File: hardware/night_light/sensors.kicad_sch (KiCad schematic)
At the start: 6 parts, among them J1 RDB223

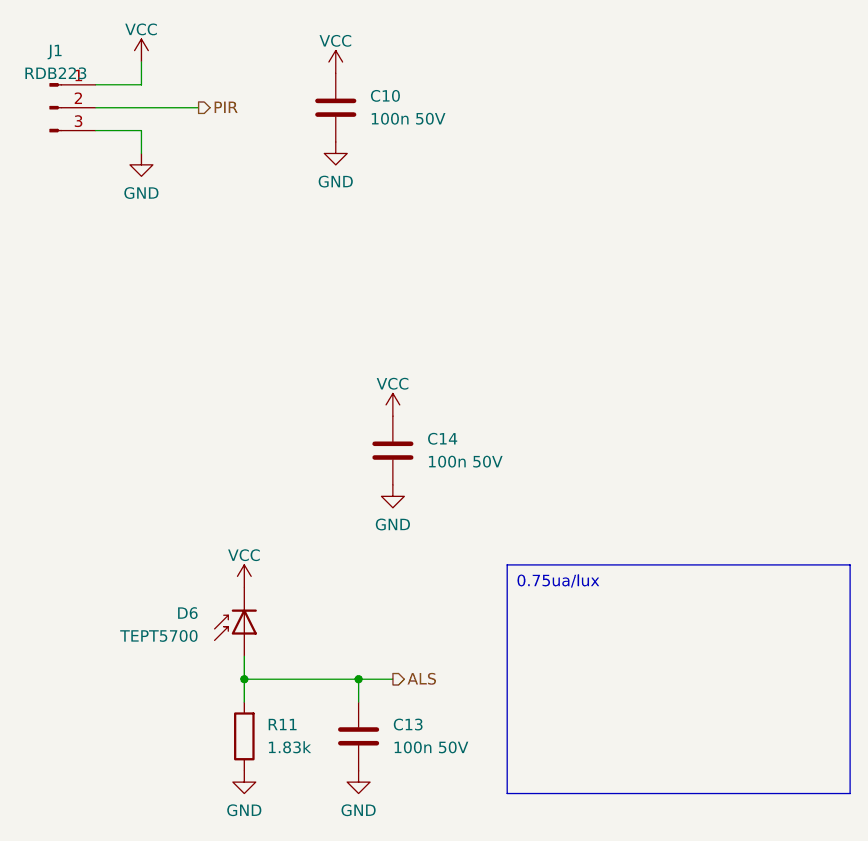
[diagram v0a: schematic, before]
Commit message: Night Light firmware
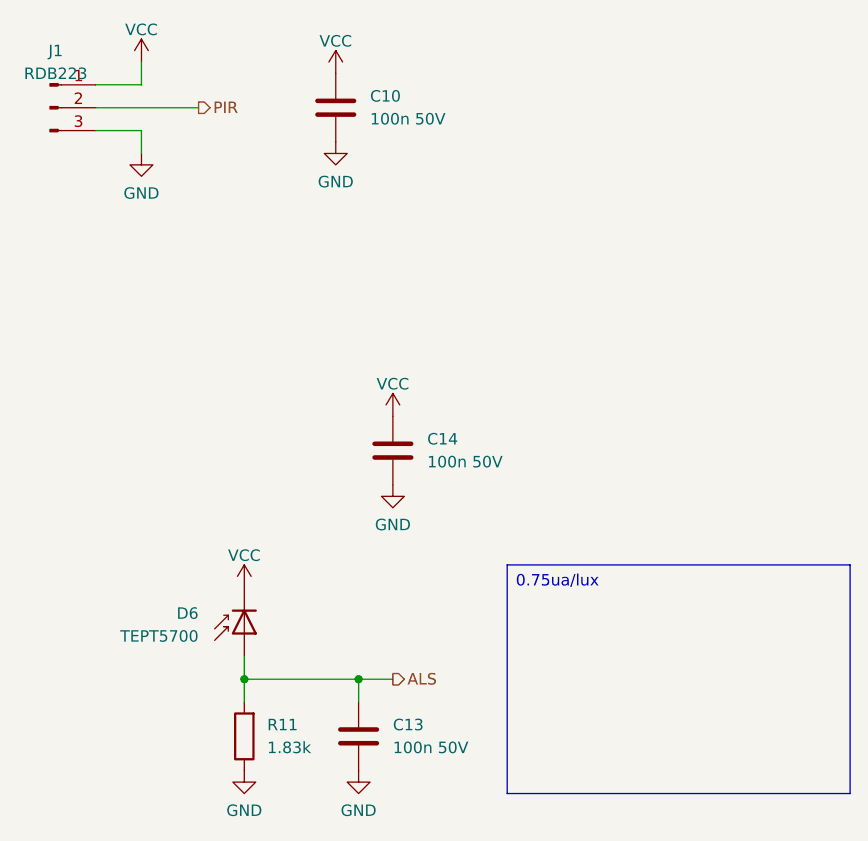
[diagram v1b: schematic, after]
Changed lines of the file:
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@@
 (kicad_sch
-	(version 20231120)
+	(version 20250114)
 	(generator "eeschema")
-	(generator_version "8.0")
+	(generator_version "9.0")
 	(paper "A4")
+	(text_box "0.75ua/lux\n"
+		(exclude_from_sim no)
+		(at 165.1 127 0)
+		(size 38.1 25.4)
+		(margins 0.9525 0.9525 0.9525 0.9525)
+		(stroke
+			(width 0)
+			(type default)
+		)
+		(fill
+			(type none)
+		)
+		(effects
+			(font
+				(size 1.27 1.27)
+			)
+			(justify left top)
+		)
+	)
 	(junction
 		(at 148.59 139.7)
@@
 		)
 	)
-	(text_box "0.75ua/lux\n"
-		(exclude_from_sim no)
-		(at 165.1 127 0)
-		(size 38.1 25.4)
-		(stroke
-			(width 0)
-			(type default)
-		)
-		(fill
-			(type none)
-		)
-		(effects
-			(font
-				(size 1.27 1.27)
-			)
-			(justify left top)
-		)
-	)
 	(hierarchical_label "ALS"
 		(shape output)
 		(at 152.4 139.7 0)
-		(fields_autoplaced yes)
 		(effects
 			(font
@@
 		(shape output)
 		(at 130.81 76.2 0)
-		(fields_autoplaced yes)
 		(effects
 			(font
